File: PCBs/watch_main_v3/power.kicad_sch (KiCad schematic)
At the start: 18 parts, among them IC201 ADP5360ACBZ-2-R7, Q201 DMP2104LP-7

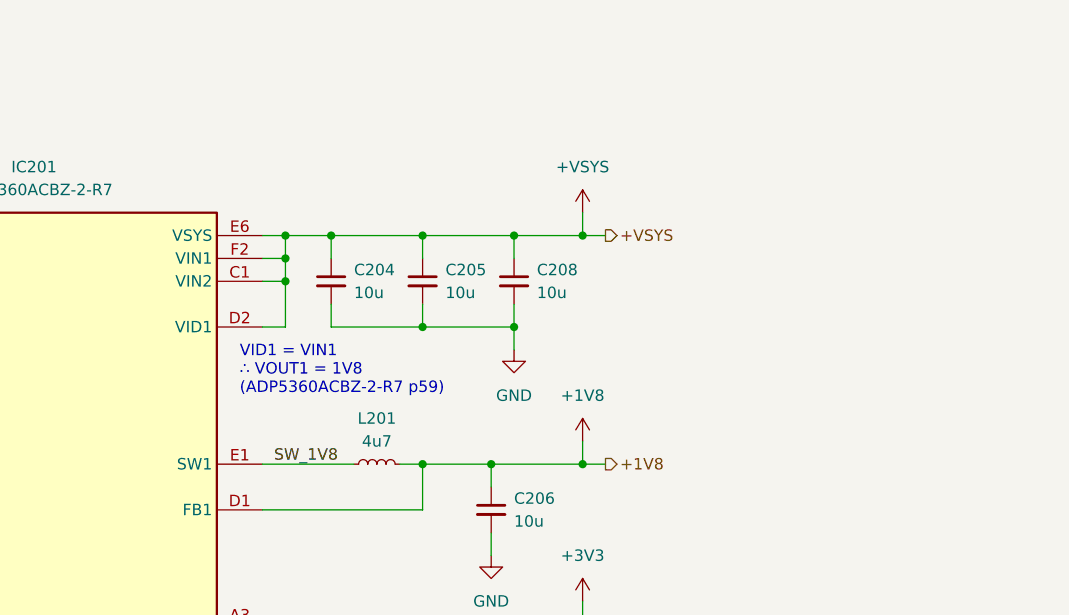
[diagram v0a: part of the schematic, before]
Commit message: PCB V3 Progress
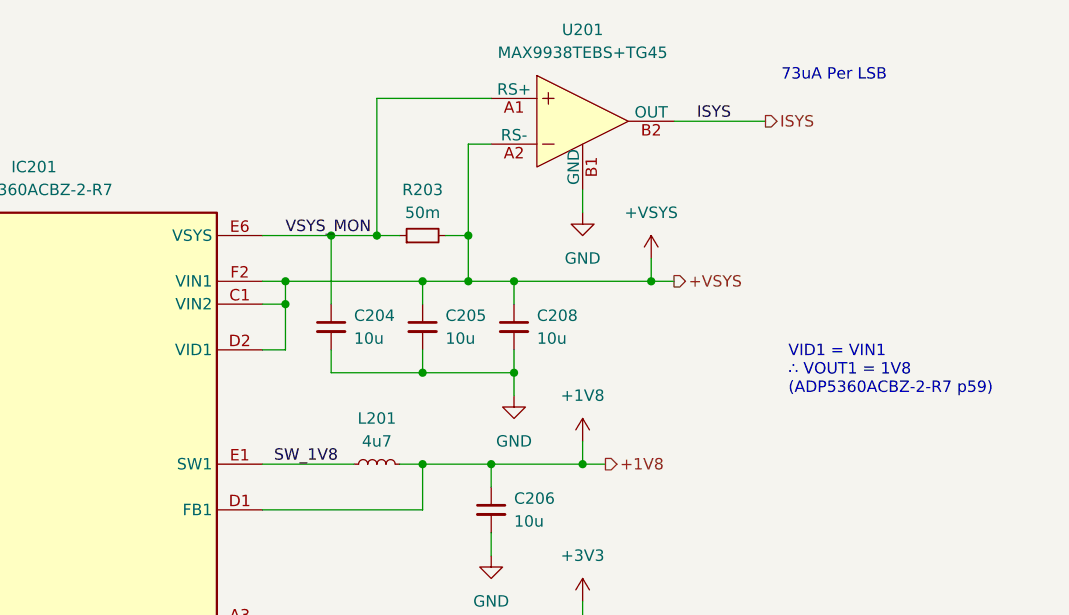
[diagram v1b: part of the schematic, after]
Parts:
- added R203: 50m, Resistor_SMD:R_0402_1005Metric, symbol Device:R_Small
- added U201: MAX9938TEBS+TG45, watch_footprints:BGA4C50P2X2_100X100X67, symbol MAX9938TEBS+TG45:MAX9938TEBS+TG45
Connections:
- net +VSYS: now also R203.2, U201.A2 (RS-); no longer C204.1, IC201.E6 (VSYS)
- net GND: now also U201.B1 (GND)
- new net ISYS: U201.B2 (OUT)
- new net VSYS_MON: C204.1, IC201.E6 (VSYS), R203.1, U201.A1 (RS+)
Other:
- note added: "73uA Per LSB"
- moved on the sheet: C204
